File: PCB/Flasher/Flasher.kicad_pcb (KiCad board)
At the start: 2 copper layers, 70 x 70 mm, 37 parts, among them J3 Reset, U1 TPS562246, U4 ESP32-S3-MINI-1

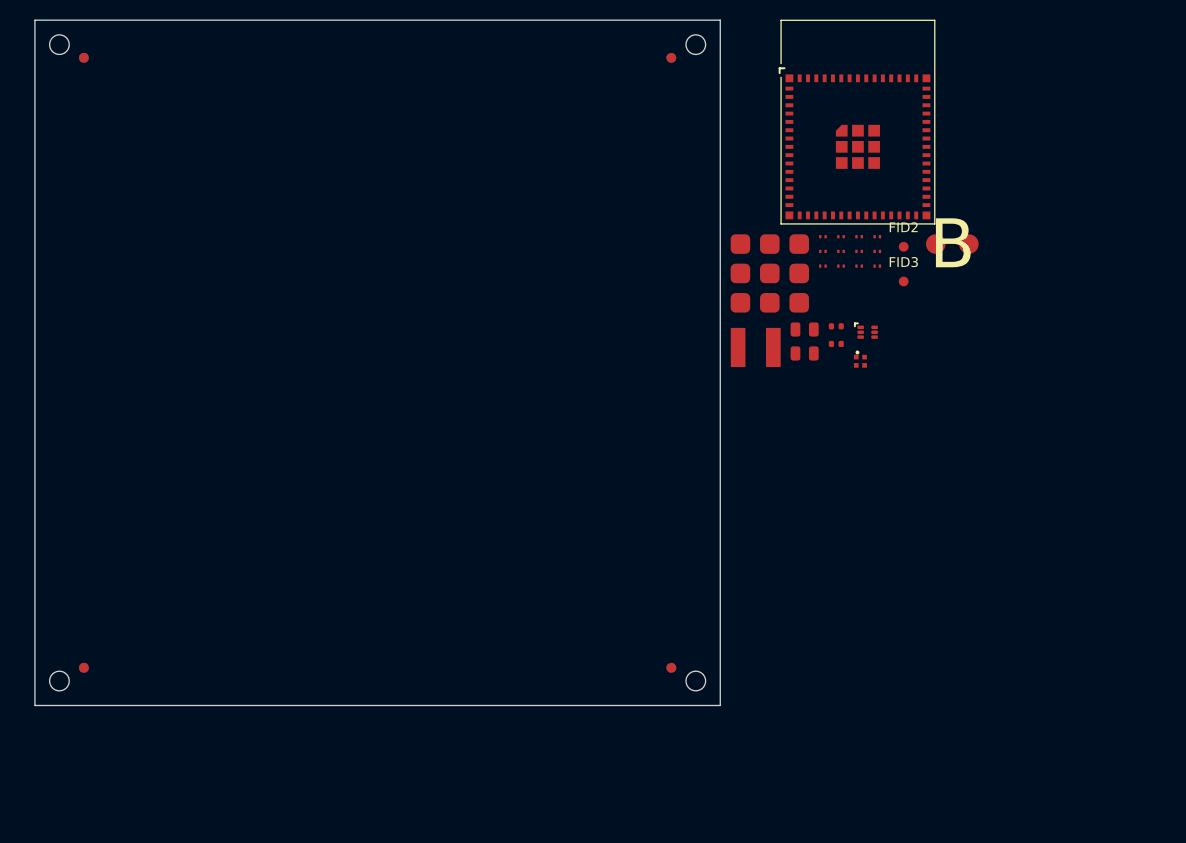
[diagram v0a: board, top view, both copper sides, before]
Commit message: Parts
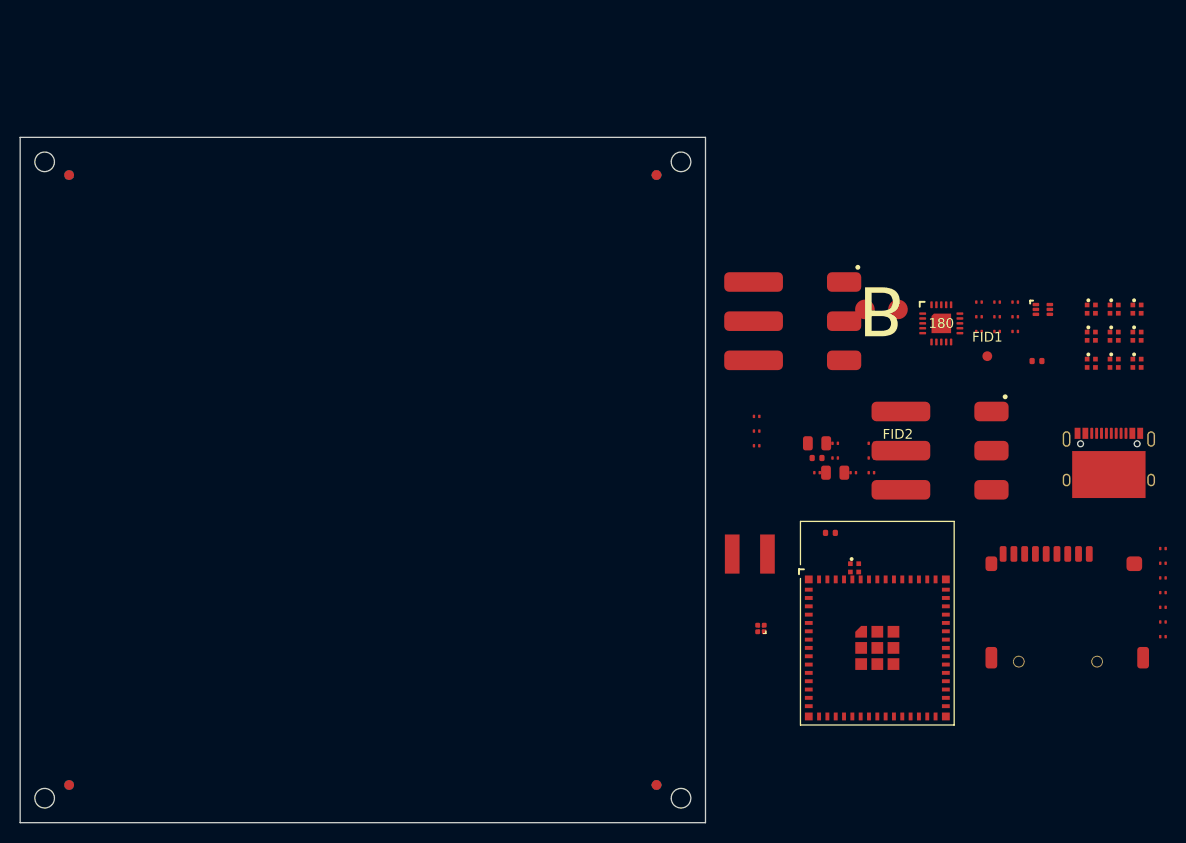
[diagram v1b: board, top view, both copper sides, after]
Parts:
- removed C17: 22uF 25V, RevK:C_0805
- removed C18: 100nF, RevK:C_0201
- removed C19: 18pF, RevK:C_0201
- removed FID3: Fiducial, Fiducial:Fiducial_1mm_Mask2mm
- removed TP10, TP2, TP3, TP4, TP5, TP6, TP7, TP8, TP9: TestPoint, RevK:PAD-2mm
- removed V5, V6: ~, RevK:VCUT70N
- added C10: 100nF, RevK:C_0201, F.Cu at (197.9, 49.8)
- added C11: 100nF, RevK:C_0201, F.Cu at (199.8, 46.8)
- added C12: 100nF, RevK:C_0201, F.Cu at (199.8, 48.3)
- added C13: 100nF, RevK:C_0402, F.Cu at (203.9, 52.8)
- added C14: 100nF, RevK:C_0201, F.Cu at (175.2, 58.5)
- added C8: 100nF, RevK:C_0201, F.Cu at (197.9, 46.8)
- added C9: 100nF, RevK:C_0201, F.Cu at (197.9, 48.3)
- added D10: XL-1010RGBC-WS2812B, RevK:SMD1010, F.Cu at (214.1, 53.1)
- added D2: XL-1010RGBC-WS2812B, RevK:SMD1010, F.Cu at (209.4, 47.5)
- added D3: XL-1010RGBC-WS2812B, RevK:SMD1010, F.Cu at (211.7, 47.5)
- added D4: XL-1010RGBC-WS2812B, RevK:SMD1010, F.Cu at (214.1, 47.5)
- added D5: XL-1010RGBC-WS2812B, RevK:SMD1010, F.Cu at (209.4, 50.3)
- added D6: XL-1010RGBC-WS2812B, RevK:SMD1010, F.Cu at (211.7, 50.3)
- added D7: XL-1010RGBC-WS2812B, RevK:SMD1010, F.Cu at (214.1, 50.3)
- added D8: XL-1010RGBC-WS2812B, RevK:SMD1010, F.Cu at (209.4, 53.1)
- added D9: XL-1010RGBC-WS2812B, RevK:SMD1010, F.Cu at (211.7, 53.1)
- added FID1: Fiducial, Fiducial:Fiducial_1mm_Mask2mm, F.Cu at (198.8, 52.4)
- added J1: Reset, RevK:AA-Pad, F.Cu at (188.0, 47.6)
- added J2: Wago, RevK:WAGO-2060-453-998-404, F.Cu at (179.6, 48.8)
- added J4: USB-C-Socket-V, RevK:USB-C-Socket-H, F.Cu at (211.2, 61.8)
- added J5: TF_PUSH, RevK:TF_PUSH, F.Cu at (206.9, 80.4)
- added R1: 150k 1%, RevK:R_0201, F.Cu at (199.8, 49.8)
- added R10: 27R, RevK:R_0201, F.Cu at (216.7, 73.5)
- added R11: 10K, RevK:R_0201, F.Cu at (216.7, 75.0)
- added R12: 10K, RevK:R_0201, F.Cu at (216.7, 76.5)
- added R13: 10K, RevK:R_0201, F.Cu at (216.7, 78.0)
- added R14: 10K, RevK:R_0201, F.Cu at (216.7, 79.5)
- added R15: 10K, RevK:R_0201, F.Cu at (216.7, 81.0)
- added R2: 10K, RevK:R_0201, F.Cu at (201.6, 46.8)
- added R4: 33k 1%, RevK:R_0201, F.Cu at (201.6, 48.3)
- added R7: 5K1, RevK:R_0201, F.Cu at (201.6, 49.8)
- added R9: 27R, RevK:R_0201, F.Cu at (216.7, 72.0)
- added U2: TPS562246, RevK:SOT-563, F.Cu at (204.5, 47.6)
- added U3: FT231XQ, RevK:QFN-20-1EP_4x4mm_P0.5mm_EP2.5x2.5mm, F.Cu at (194.1, 49.0)
- added V1: ~, RevK:VCUT70N, F.Cu at (209.4, 37.2)
- added V2: ~, RevK:VCUT70N, F.Cu at (209.4, 39.7)
- C1: value 100nF -> 22uF 25V; footprint RevK:C_0201 -> RevK:C_0805
- C15: value 47uF 6V -> 100nF; footprint RevK:C_0805 -> RevK:C_0201
- C16: value 100nF 25V -> 100nF; footprint RevK:C_0402 -> RevK:C_0201
- C2: value 100nF -> 100nF 25V; footprint RevK:C_0201 -> RevK:C_0402
- C4: value 100nF -> 1uF
- C6: value 1uF -> 18pF
- C7: value 100nF -> 47uF 6V; footprint RevK:C_0201 -> RevK:C_0805
- J3: value Reset -> Wago; footprint RevK:AA-Pad -> RevK:WAGO-2060-453-998-404
- R3: value 10K -> 150k 1%
- R5, R6: value 150k 1% -> 10K
- R8: value 33k 1% -> 5K1
- U1: value TPS562246 -> ESP32-S3-MINI-1; footprint RevK:SOT-563 -> RevK:ESP32-S3-MINI-1
- U4: value ESP32-S3-MINI-1 -> TPS22916CNYFPR; footprint RevK:ESP32-S3-MINI-1 -> RevK:WCSP-4-0.78x0.78
- moved V3 96.4 mm to (209.5, 32.0)
- moved V4 96.4 mm to (209.5, 34.4)
- moved U4 50.2 mm to (175.7, 80.2)
- moved U1 32.3 mm to (187.6, 82.2)
- moved C3 21.1 mm to (182.8, 70.4)
- moved C1 21.1 mm to (181.4, 61.2)
- moved C2 21.1 mm to (181.4, 62.8)
- moved C4 21.1 mm to (181.4, 64.2)
- moved C5 21.1 mm to (183.2, 61.2)
- moved C6 21.1 mm to (183.2, 62.8)
- moved C7 21.1 mm to (183.2, 64.2)
- moved D1 21.1 mm to (185.2, 74.0)
- moved FID2 21.1 mm to (189.6, 62.3)
- moved J3 21.1 mm to (194.6, 62.0)
- moved L1 21.1 mm to (174.5, 72.6)
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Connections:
- C1 pad 1: GND -> DC
- C1 pad 2: +3.3V -> GND
- C16 pad 1: DC -> +3.3V
- C2 pad 1: GND -> DC
- C2 pad 2: +3.3V -> GND
- C4 pad 1: GND -> RST
- C4 pad 2: +3.3V -> GND
- C5 pad 1: GND -> BST
- C5 pad 2: +3.3V -> SW
- C6 pad 1: RST -> FB
- C6 pad 2: GND -> +3.3V
- C7 pad 1: GND -> +3.3V
- C7 pad 2: +3.3V -> GND
- D1 pad 1: unconnected-(D1-O-Pad1) -> Net-(D1-O)
- J3 pad 1: GND -> Net-(J3-Pin_1)
- J3 pad 2: Net-(J3-Pin_2) -> Net-(J2-Pin_3)
- R3 pad 2: RST -> FB
- R5 pad 1: EN -> +3.3V
- R5 pad 2: DC -> SDCD
- R6 pad 2: FB -> SDDAT1
- R8 pad 1: FB -> GND
- R8 pad 2: GND -> Net-(J4-CC2)
- U1 pad 1: DC -> GND
- U1 pad 2: SW -> GND
- U1 pad 3: GND -> +3.3V
- U1 pad 4: BST -> GPIO0
- U1 pad 5: EN -> unconnected-(U1-GPIO1-Pad5)
- U1 pad 6: FB -> unconnected-(U1-GPIO2-Pad6)
